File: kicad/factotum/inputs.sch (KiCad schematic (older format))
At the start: 40 parts, among them J21 Conn_01x05_Male, J22 Conn_01x08_Male, J4 Conn_01x05_Female, J5 VOCT, J6 Conn_01x08_Female, J7 RST, J8 CLK, P1 10k, P2 10k, P3 10k, P4 10k, SW1 MODE_SW, U4 MCP6004, U5 ADC128S022

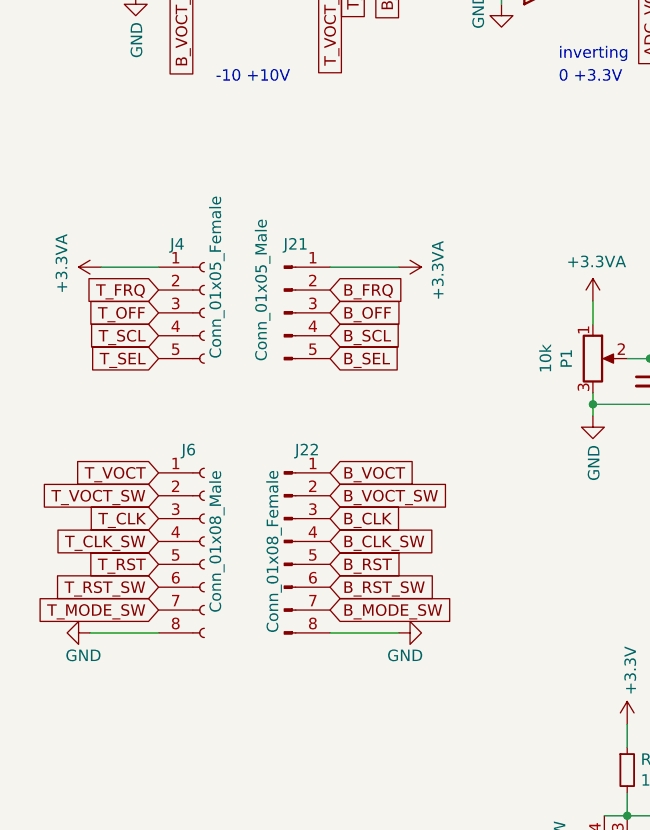
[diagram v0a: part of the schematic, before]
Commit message: more work on routing
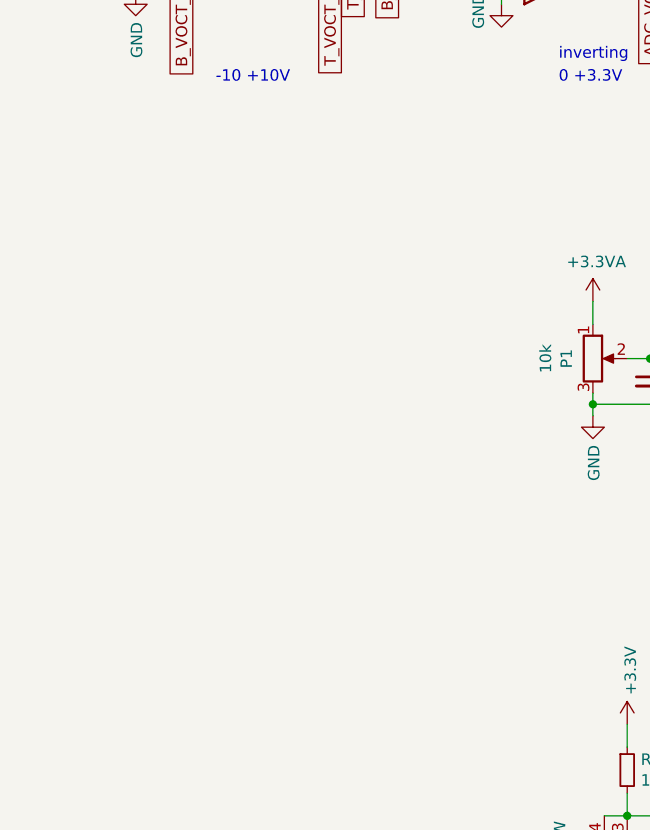
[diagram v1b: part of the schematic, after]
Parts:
- removed J21: Conn_01x05_Male, Connector_PinHeader_2.54mm:PinHeader_1x05_P2.54mm_Vertical, symbol Connector:Conn_01x05_Male
- removed J22: Conn_01x08_Male, Connector_PinHeader_2.54mm:PinHeader_1x08_P2.54mm_Vertical, symbol Connector:Conn_01x08_Male
- removed J4: Conn_01x05_Female, Connector_PinSocket_2.54mm:PinSocket_1x05_P2.54mm_Vertical, symbol Connector:Conn_01x05_Female
- removed J6: Conn_01x08_Female, Connector_PinSocket_2.54mm:PinSocket_1x08_P2.54mm_Vertical, symbol Connector:Conn_01x08_Female
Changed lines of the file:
@@
 	1    0    0    -1
 $EndComp
-Text GLabel 1850 3100 2    50   Input ~ 0
-B_FRQ
 $Comp
 L Device:R_POT FRQ?
@@
 Wire Wire Line
 	4150 3600 4150 3700
-Text GLabel 1850 3400 2    50   Input ~ 0
-B_SEL
 $Comp
 L Device:R_POT FRQ?
@@
 Wire Wire Line
 	5300 3600 5300 3700
-Text GLabel 1850 3300 2    50   Input ~ 0
-B_SCL
 $Comp
 L Device:R_POT FRQ?
@@
 Wire Wire Line
 	6450 3600 6450 3700
-Text GLabel 1850 3200 2    50   Input ~ 0
-B_OFF
 Text GLabel 5000 4800 0    50   Input ~ 0
 B_FRQ
@@
 Text GLabel 3350 3400 2    50   Input ~ 0
 T_FRQ
-Text GLabel 1100 3100 0    50   Input ~ 0
-T_FRQ
 Wire Wire Line
 	3150 3400 3250 3400
@@
 	4400 3600 4150 3600
 Text GLabel 4500 3400 2    50   Input ~ 0
-T_SEL
-Text GLabel 1100 3400 0    50   Input ~ 0
 T_SEL
 Connection ~ 5550 3400
@@
 Text GLabel 5650 3400 2    50   Input ~ 0
 T_OFF
-Text GLabel 1100 3200 0    50   Input ~ 0
-T_OFF
-Text GLabel 1100 3300 0    50   Input ~ 0
-T_SCL
 Text GLabel 1950 1550 3    50   Input ~ 0
 T_VOCT
-Text GLabel 1100 3900 0    50   Input ~ 0
-T_VOCT
 Text GLabel 2100 1550 3    50   Input ~ 0
-B_VOCT
-Text GLabel 1850 3900 2    50   Input ~ 0
 B_VOCT
 Text GLabel 4850 1550 3    50   Input ~ 0
@@
 Text GLabel 8050 1550 3    50   Input ~ 0
 B_CLK
-Text GLabel 1100 4300 0    50   Input ~ 0
-T_RST
-Text GLabel 1850 4100 2    50   Input ~ 0
-B_CLK
-Text GLabel 1100 4100 0    50   Input ~ 0
-T_CLK
-Text GLabel 1850 4300 2    50   Input ~ 0
-B_RST
-Text GLabel 1850 4500 2    50   Input ~ 0
-B_MODE_SW
-Text GLabel 1100 4500 0    50   Input ~ 0
-T_MODE_SW
-$Comp
-L power:+3.3VA #PWR030
-U 1 1 5FE170F7
-P 850 3000
-F 0 "#PWR030" H 850 2850 50  0001 C CNN
-F 1 "+3.3VA" H 865 3173 50  0000 C CNN
-F 2 "" H 850 3000 50  0001 C CNN
-F 3 "" H 850 3000 50  0001 C CNN
-	1    850  3000
-	0    -1   -1   0
-$EndComp
-$Comp
-L power:+3.3VA #PWR034
-U 1 1 5FE18226
-P 2150 3000
-F 0 "#PWR034" H 2150 2850 50  0001 C CNN
-F 1 "+3.3VA" H 2165 3173 50  0000 C CNN
-F 2 "" H 2150 3000 50  0001 C CNN
-F 3 "" H 2150 3000 50  0001 C CNN
-	1    2150 3000
-	0    1    1    0
-$EndComp
-$Comp
-L power:GND #PWR?
-U 1 1 5FE18FBB
-P 800 4600
-AR Path="/5FE18FBB" Ref="#PWR?"  Part="1"
-AR Path="/606FF2F2/5FE18FBB" Ref="#PWR029"  Part="1"
-F 0 "#PWR029" H 800 4350 50  0001 C CNN
-F 1 "GND" V 900 4650 50  0000 R CNN
-F 2 "" H 800 4600 50  0001 C CNN
-F 3 "" H 800 4600 50  0001 C CNN
-	1    800  4600
-	0    1    1    0
-$EndComp
-$Comp
-L power:GND #PWR?
-U 1 1 5FE1CBFF
-P 2150 4600
-AR Path="/5FE1CBFF" Ref="#PWR?"  Part="1"
-AR Path="/606FF2F2/5FE1CBFF" Ref="#PWR035"  Part="1"
-F 0 "#PWR035" H 2150 4350 50  0001 C CNN
-F 1 "GND" V 2050 4650 50  0000 R CNN
-F 2 "" H 2150 4600 50  0001 C CNN
-F 3 "" H 2150 4600 50  0001 C CNN
-	1    2150 4600
-	0    -1   -1   0
-$EndComp
-Wire Wire Line
-	850  3000 1100 3000
-Wire Wire Line
-	1850 3000 2150 3000
 Wire Wire Line
 	4750 1550 4850 1550
@@
 Wire Wire Line
 	6950 4900 6950 5000
-$Comp
-L Connector:Conn_01x05_Female J4
-U 1 1 5FD0067F
-P 1300 3200
-F 0 "J4" H 1150 3500 50  0000 L CNN
-F 1 "Conn_01x05_Female" V 1350 3000 50  0000 L CNN
-F 2 "Connector_PinSocket_2.54mm:PinSocket_1x05_P2.54mm_Vertical" H 1300 3200 50  0001 C CNN
-F 3 "~" H 1300 3200 50  0001 C CNN
-	1    1300 3200
-	1    0    0    -1
-$EndComp
-$Comp
-L Connector:Conn_01x05_Male J21
-U 1 1 5FD01CE2
-P 1650 3200
-F 0 "J21" H 1700 3500 50  0000 C CNN
-F 1 "Conn_01x05_Male" V 1550 3300 50  0000 C CNN
-F 2 "Connector_PinHeader_2.54mm:PinHeader_1x05_P2.54mm_Vertical" H 1650 3200 50  0001 C CNN
-F 3 "~" H 1650 3200 50  0001 C CNN
-	1    1650 3200
-	1    0    0    -1
-$EndComp
-Wire Wire Line
-	2150 4600 1850 4600
-Wire Wire Line
-	1100 4600 800  4600
 Wire Wire Line
 	1850 1450 1950 1450
@@
 Text GLabel 7800 1650 3    50   Input ~ 0
 T_CLK_SW
-$Comp
-L Connector:Conn_01x08_Female J6
-U 1 1 600A03D9
-P 1300 4200
-F 0 "J6" H 1200 4600 50  0000 L CNN
-F 1 "Conn_01x08_Female" V 1600 3800 50  0000 L CNN
-F 2 "Connector_PinSocket_2.54mm:PinSocket_1x08_P2.54mm_Vertical" H 1300 4200 50  0001 C CNN
-F 3 "~" H 1300 4200 50  0001 C CNN
-	1    1300 4200
-	1    0    0    -1
-$EndComp
-$Comp
-L Connector:Conn_01x08_Male J22
-U 1 1 600A30A6
-P 1650 4200
-F 0 "J22" H 1750 4600 50  0000 C CNN
-F 1 "Conn_01x08_Male" V 1350 4200 50  0000 C CNN
-F 2 "Connector_PinHeader_2.54mm:PinHeader_1x08_P2.54mm_Vertical" H 1650 4200 50  0001 C CNN
-F 3 "~" H 1650 4200 50  0001 C CNN
-	1    1650 4200
-	1    0    0    -1
-$EndComp
-Text GLabel 1100 4000 0    50   Input ~ 0
-T_VOCT_SW
-Text GLabel 1100 4200 0    50   Input ~ 0
-T_CLK_SW
-Text GLabel 1100 4400 0    50   Input ~ 0
-T_RST_SW
-Text GLabel 1850 4000 2    50   Input ~ 0
-B_VOCT_SW
-Text GLabel 1850 4200 2    50   Input ~ 0
-B_CLK_SW
-Text GLabel 1850 4400 2    50   Input ~ 0
-B_RST_SW
 NoConn ~ 6050 4200
 $EndSCHEMATC
